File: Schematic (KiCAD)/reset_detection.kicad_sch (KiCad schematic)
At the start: 54 parts, among them P29 INVERT, X15 INVERT

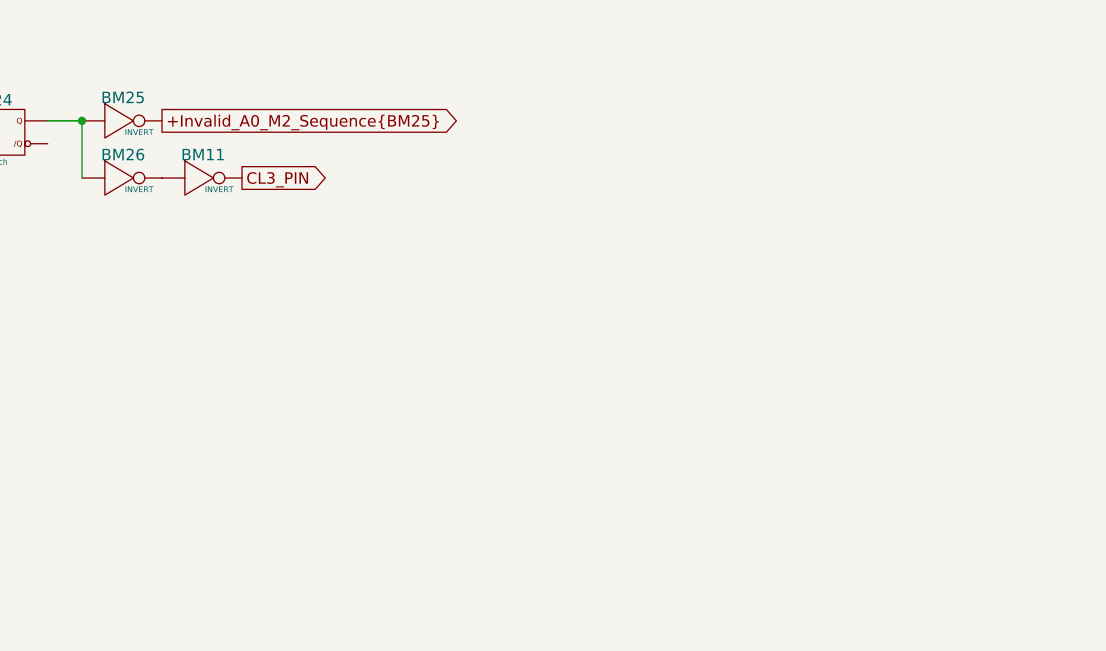
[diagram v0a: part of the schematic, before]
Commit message: Schematic and SVG Updates
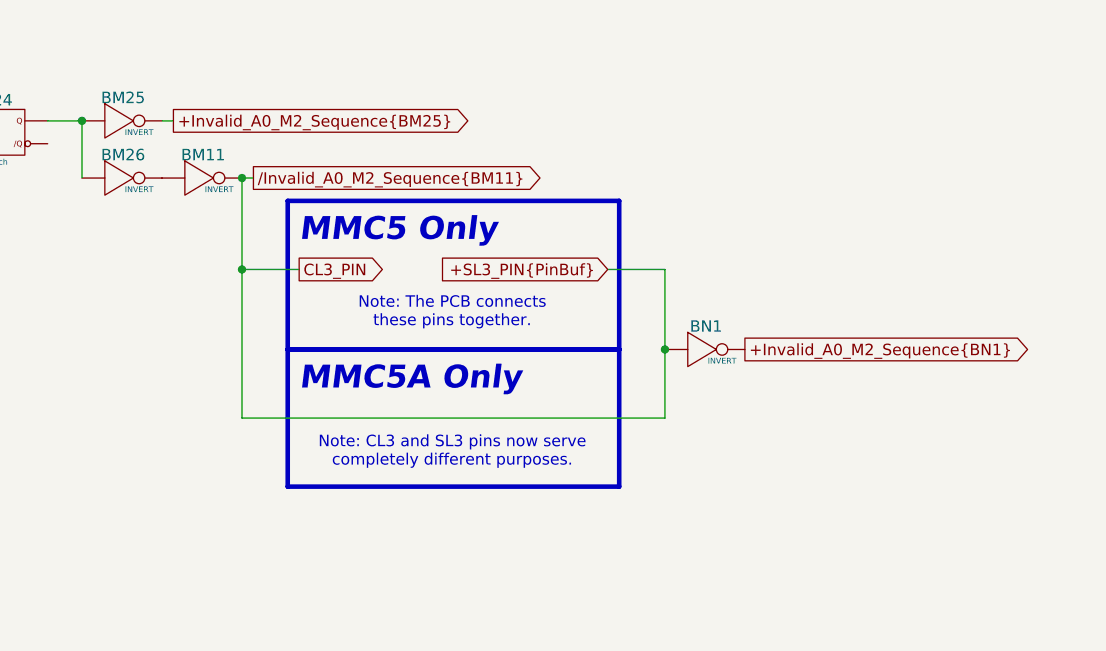
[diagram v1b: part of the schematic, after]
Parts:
- added BN1: INVERT, symbol MMC5:INVERT
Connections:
- net at OSC4. (X): now also OSC3. (X); no longer OSC5. (X)
- net at OSC3. (X): now also OSC2. (X); no longer OSC4. (X)
- net at D41. (X): now also D42. (X); no longer D40. (X)
- net at BM23. (X): now also BM24. (/Q); no longer BM22(a). (/Q)
- net at BM24. (/Q): no longer BM23. (X)
- net at RAX3. (/Q6): now also RAX2. (X); no longer RAX1. (X)
- net at RAX4. (X): now also RAX2. (X); no longer RAX3. (/Q6)
- net at RAX7. (X): now also RAX6. (X); no longer RAX3. (/Q6)
- net at RAX5. (X): now also RAX14. (X), RAX9. (X); no longer RAX6. (X)
- net at RAX13. (X), RAX15. (X): now also RAX16. (X)
- net CL3_PIN renamed +SL3_PIN{PinBuf}
- net +SL3_PIN{PinBuf}: now also BN1. (X)
- new net: BM24. (/Q), BM25. (X), BM26. (X)
- new net: BM22(b). (/Q), BM22(c). (X)
- new net: OSC4. (X), OSC5. (X)
- new net: D40. (X), D41. (X)
- new net: BM22(a). (/Q), BM23. (X)
- new net: BM22(b). (/Q), BM23. (X)
- new net: OSC1. (X), OSC3. (X)
- new net: RAX1. (X), RAX3. (/Q6)
- new net: BM18. (X), BM19. (X), BM20. (X)
- new net: BM13,14,15,16,17. (Q3), BM19. (X) (x3)
- new net: RAX3. (/Q6), RAX4. (X)
- new net: RAX3. (/Q6), RAX7. (X)
- new net: B101. (X), B102. (X)
- new net: RAX5. (X), RAX6. (X)
- new net: RAX6. (X), RAX7. (X), RAX8. (X)
- new net: RAX10. (X), RAX13. (X), RAX9. (X)
- new net: RAX13. (X), RAX15. (X)
- new net: RAX12. (X), RAX13. (X)
- new net: BM13,14,15,16,17. (Q3), BM18. (X)
- new net +Invalid_A0_M2_Sequence{BN1}: BN1. (X)
- now unconnected: BM24. (/Q)
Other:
- note added: "MMC5 Only"
- note added: "MMC5A Only"
- note added: "Note: CL3 and SL3 pins now serve completely different purposes."
- note added: "Note: The PCB connects these pins together."
